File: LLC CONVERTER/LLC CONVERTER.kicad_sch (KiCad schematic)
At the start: 19 parts, among them IC1 UCC256601DDBR, J1 SPADE, J2 SPADE

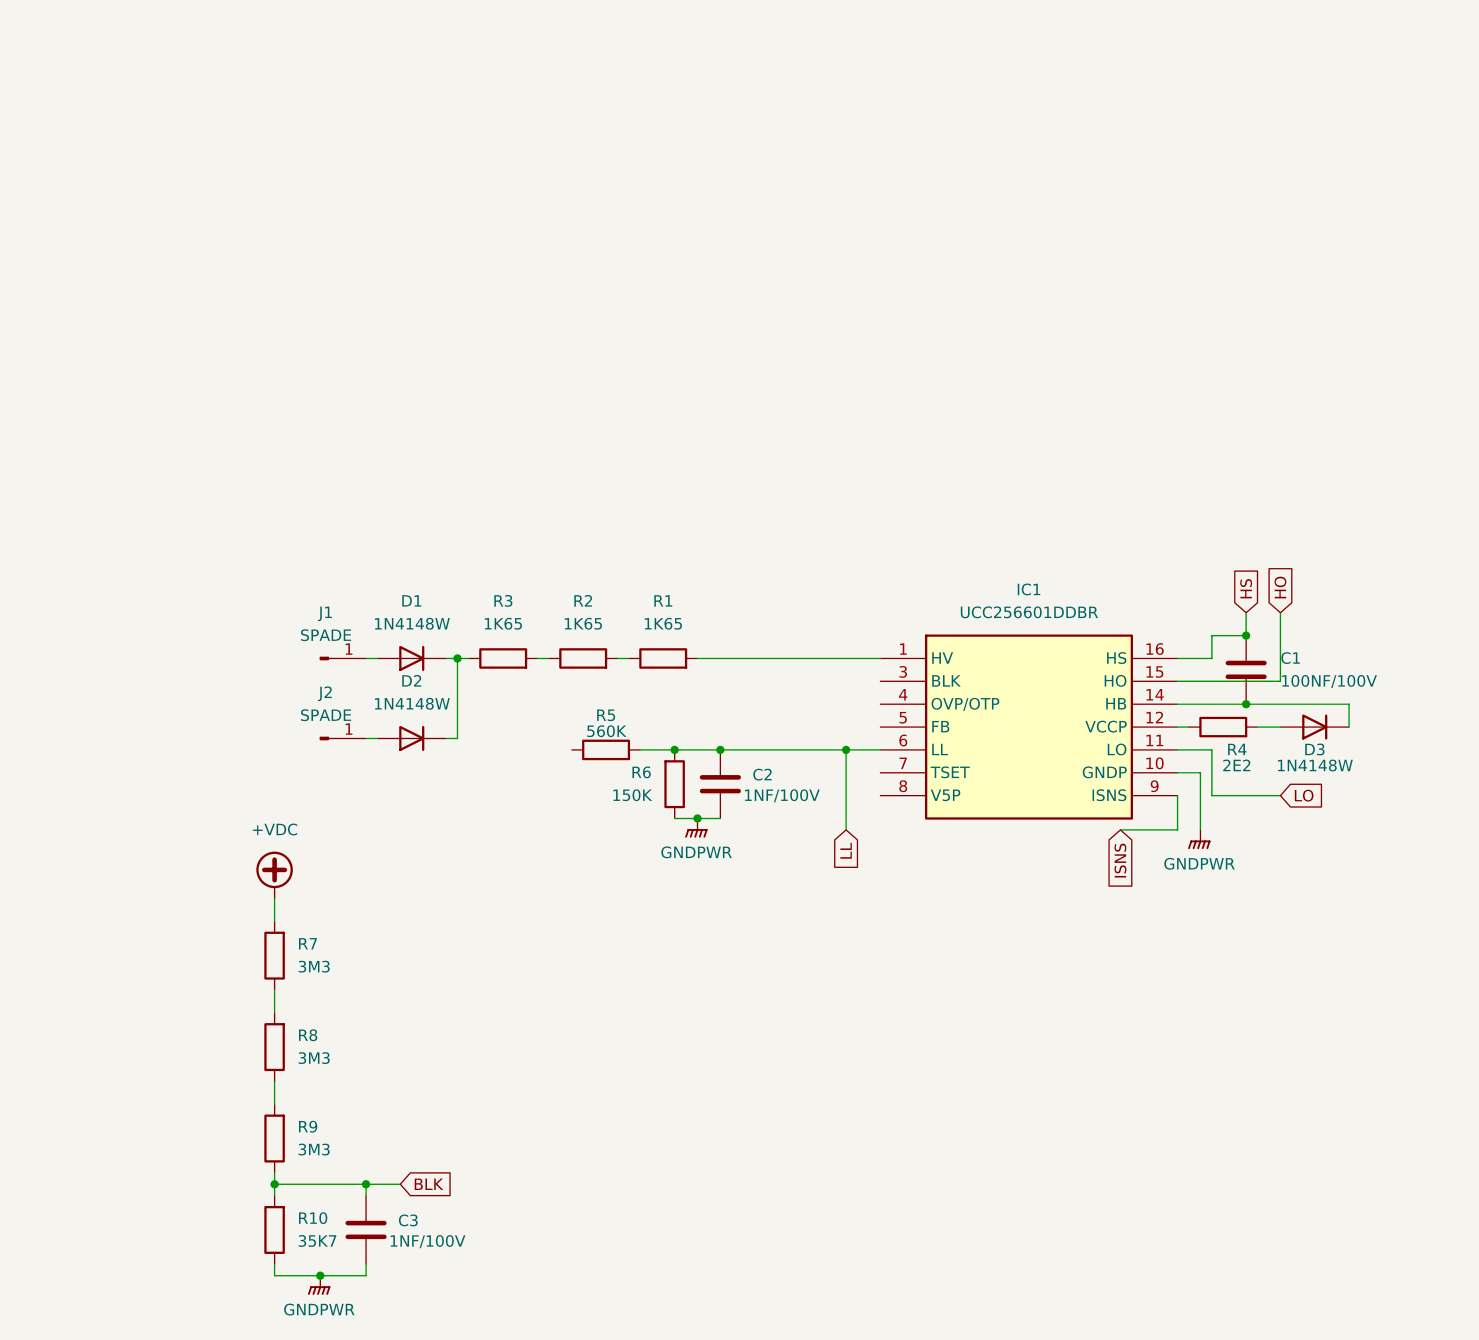
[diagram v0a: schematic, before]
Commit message: first commit
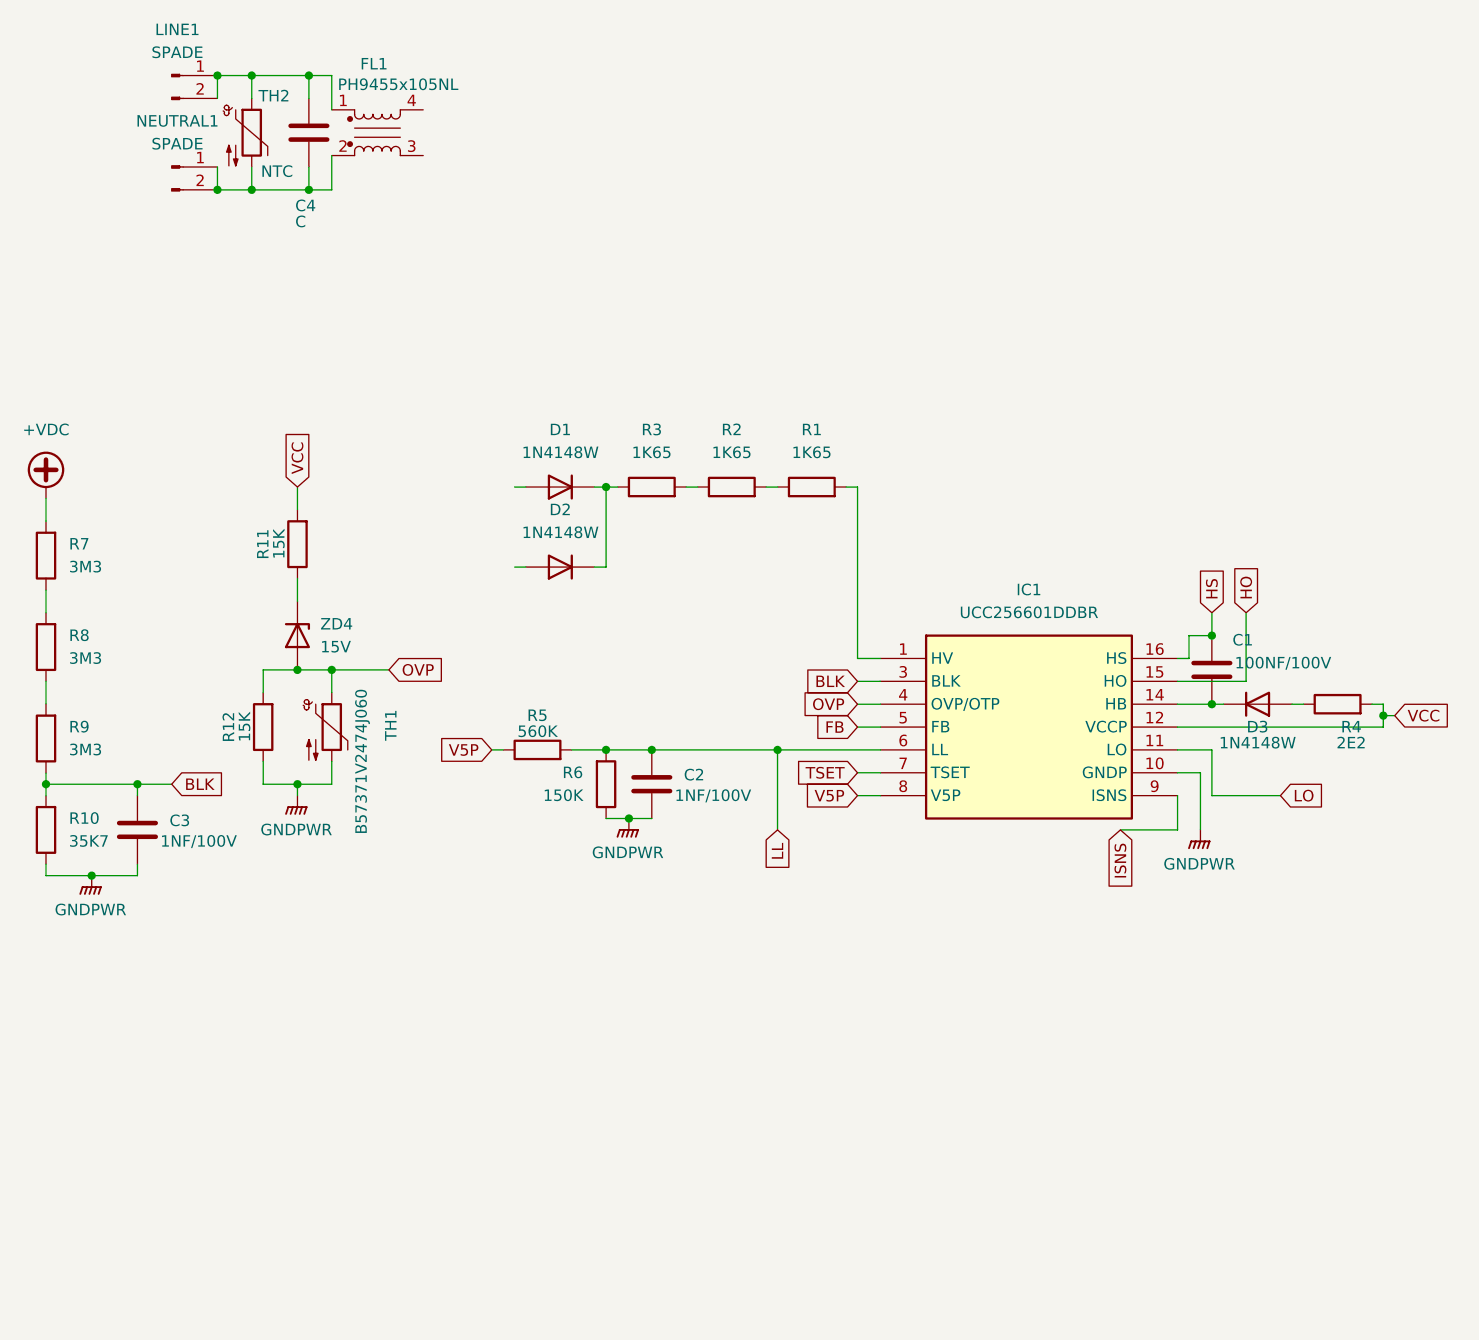
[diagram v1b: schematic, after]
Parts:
- added C4: C, Capacitor_THT:C_Rect_L13.5mm_W5.0mm_P10.00mm_FKS3_FKP3_MKS4, symbol Device:C
- added FL1: PH9455x105NL, Inductor_THT:L_CommonMode_PulseElectronics_PH9455x105NL_1, symbol Filter:Choke_CommonMode_PulseElectronics_PH9455x105NL
- added R11, R12: 15K, Resistor_SMD:R_1206_3216Metric, symbol Device:R
- added TH1: B57371V2474J060, Resistor_SMD:R_0603_1608Metric_Pad0.98x0.95mm_HandSolder, symbol Device:Thermistor_NTC
- added TH2: NTC, Resistor_THT:R_Bare_Metal_Element_L12.4mm_W4.8mm_P11.40mm, symbol Device:Thermistor_NTC
- added ZD4: 15V, Diode_SMD:D_SOD-123, symbol Device:D_Zener
- LINE1: renamed from J1; symbol Connector:Conn_01x01_Pin -> Connector:Conn_01x02_Pin
- NEUTRAL1: renamed from J2; symbol Connector:Conn_01x01_Pin -> Connector:Conn_01x02_Pin
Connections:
- net BLK: now also IC1.3 (BLK)
- net GNDPWR: now also R12.1, TH1.2
- net at D1.2 (A): no longer LINE1.1 (Pin_1)
- net V5P: now reaches R5.1
- net V5P: now also IC1.8 (V5P)
- net at NEUTRAL1.1 (Pin_1): now also NEUTRAL1.2 (Pin_2), C4.2, FL1.2, TH2.2; no longer D2.2 (A)
- net at D3.2 (A): now also R4.1; no longer R4.2
- net VCC: now reaches IC1.12 (VCCP)
- net VCC: now also R4.2, R11.2; no longer R4.1
- net OVP: now reaches IC1.4 (OVP/OTP)
- net OVP: now also R12.2, TH1.1, ZD4.2 (A)
- net FB: now reaches IC1.5 (FB)
- net TSET: now reaches IC1.7 (TSET)
- new net: C4.1, FL1.1, LINE1.1 (Pin_1), LINE1.2 (Pin_2), TH2.1
- new net: R11.1, ZD4.1 (K)
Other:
- moved on the sheet: C1, C2, C3, D1, D2, D3, R1, R10, R2, R3, R4, R5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
